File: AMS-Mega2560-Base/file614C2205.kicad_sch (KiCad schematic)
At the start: 5 parts, among them IC1 CD74HC4050ME4, IC2 CD74HC4050ME4, J6 Conn_01x03, J7 Conn_01x08

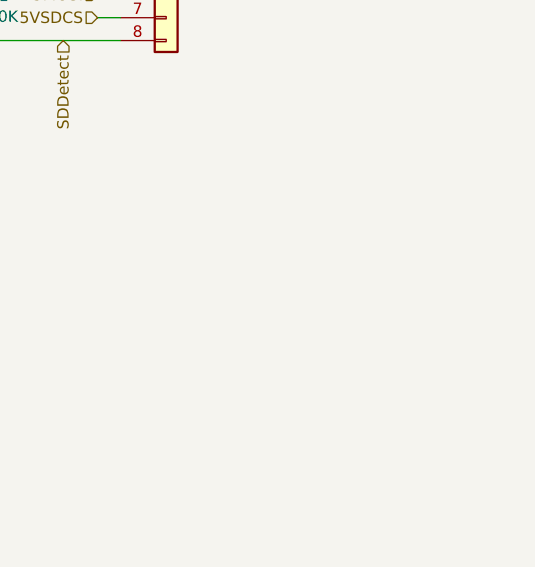
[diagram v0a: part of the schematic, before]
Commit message: BaseBoard fixes and updates. doing schematic work.
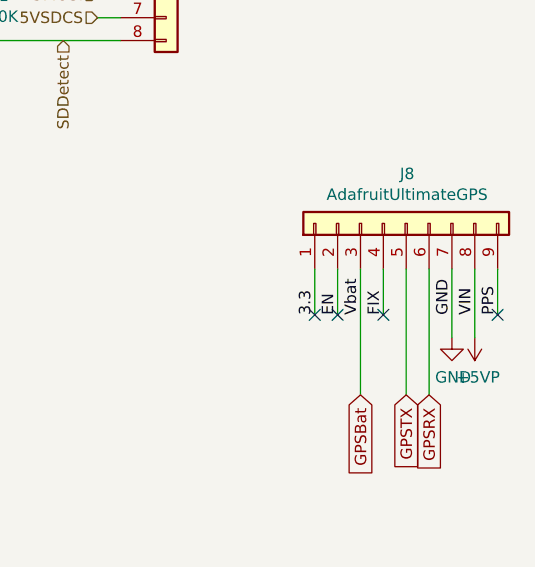
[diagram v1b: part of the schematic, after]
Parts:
- added J8: AdafruitUltimateGPS, Connector_PinSocket_2.54mm:PinSocket_1x09_P2.54mm_Vertical, symbol Connector_Generic:Conn_01x09
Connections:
- net +5VP: now also J8.8 (Pin_8)
- net GND: now also J8.7 (Pin_7)
- new net 3.3: J8.1 (Pin_1)
- new net EN: J8.2 (Pin_2)
- new net FIX: J8.4 (Pin_4)
- new net GPSBat: J8.3 (Pin_3)
- new net GPSRX: J8.6 (Pin_6)
- new net GPSTX: J8.5 (Pin_5)
- new net PPS: J8.9 (Pin_9)
- no-connect marks 7 -> 11
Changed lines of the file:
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@@
   (no_connect (at 205.74 59.69))
   (no_connect (at 81.28 45.72))
+  (no_connect (at 247.65 105.41))
   (no_connect (at 81.28 118.11))
+  (no_connect (at 227.33 105.41))
   (no_connect (at 81.28 110.49))
   (no_connect (at 81.28 38.1))
+  (no_connect (at 234.95 105.41))
+  (no_connect (at 229.87 105.41))
   (wire (pts (xy 49.53 107.95) (xy 53.34 107.95))
     (stroke (width 0) (type default) (color 0 0 0 0))
   )
+  (wire (pts (xy 227.33 105.41) (xy 227.33 100.33))
+    (stroke (width 0) (type default) (color 0 0 0 0))
+  )
   (wire (pts (xy 200.66 62.23) (xy 205.74 62.23))
     (stroke (width 0) (type default) (color 0 0 0 0))
@@
     (stroke (width 0) (type default) (color 0 0 0 0))
   )
+  (wire (pts (xy 237.49 100.33) (xy 237.49 114.3))
+    (stroke (width 0) (type default) (color 0 0 0 0))
+  )
   (wire (pts (xy 86.36 113.03) (xy 81.28 113.03))
     (stroke (width 0) (type default) (color 0 0 0 0))
@@
     (stroke (width 0) (type default) (color 0 0 0 0))
   )
+  (wire (pts (xy 232.41 100.33) (xy 232.41 114.3))
+    (stroke (width 0) (type default) (color 0 0 0 0))
+  )
   (wire (pts (xy 53.34 40.64) (xy 50.8 40.64))
     (stroke (width 0) (type default) (color 0 0 0 0))
@@
     (stroke (width 0) (type default) (color 0 0 0 0))
   )
+  (wire (pts (xy 247.65 105.41) (xy 247.65 100.33))
+    (stroke (width 0) (type default) (color 0 0 0 0))
+  )
   (wire (pts (xy 205.74 57.15) (xy 204.47 57.15))
     (stroke (width 0) (type default) (color 0 0 0 0))
@@
     (stroke (width 0) (type default) (color 0 0 0 0))
   )
+  (wire (pts (xy 240.03 100.33) (xy 240.03 114.3))
+    (stroke (width 0) (type default) (color 0 0 0 0))
+  )
   (wire (pts (xy 53.34 102.87) (xy 53.34 97.79))
     (stroke (width 0) (type default) (color 0 0 0 0))
   )
+  (wire (pts (xy 242.57 107.95) (xy 242.57 100.33))
+    (stroke (width 0) (type default) (color 0 0 0 0))
+  )
+  (wire (pts (xy 245.11 107.95) (xy 245.11 100.33))
+    (stroke (width 0) (type default) (color 0 0 0 0))
+  )
   (wire (pts (xy 50.8 48.26) (xy 53.34 48.26))
     (stroke (width 0) (type default) (color 0 0 0 0))
@@
     (stroke (width 0) (type default) (color 0 0 0 0))
   )
+  (wire (pts (xy 229.87 105.41) (xy 229.87 100.33))
+    (stroke (width 0) (type default) (color 0 0 0 0))
+  )
   (wire (pts (xy 85.09 50.8) (xy 81.28 50.8))
     (stroke (width 0) (type default) (color 0 0 0 0))
   )
+  (wire (pts (xy 234.95 105.41) (xy 234.95 100.33))
+    (stroke (width 0) (type default) (color 0 0 0 0))
+  )
   (wire (pts (xy 96.52 101.6) (xy 102.87 101.6))
     (stroke (width 0) (type default) (color 0 0 0 0))
+  )
+  (label "GND" (at 242.57 105.41 90)
+    (effects (font (size 1.27 1.27)) (justify left bottom))
+  )
+  (label "VIN" (at 245.11 105.41 90)
+    (effects (font (size 1.27 1.27)) (justify left bottom))
+  )
+  (label "FIX" (at 234.95 105.41 90)
+    (effects (font (size 1.27 1.27)) (justify left bottom))
+  )
+  (label "PPS" (at 247.65 105.41 90)
+    (effects (font (size 1.27 1.27)) (justify left bottom))
+  )
+  (label "Vbat" (at 232.41 105.41 90)
+    (effects (font (size 1.27 1.27)) (justify left bottom))
+  )
+  (label "EN" (at 229.87 105.41 90)
+    (effects (font (size 1.27 1.27)) (justify left bottom))
+  )
+  (label "3.3" (at 227.33 105.41 90)
+    (effects (font (size 1.27 1.27)) (justify left bottom))
+  )
+  (global_label "GPSTX" (shape input) (at 237.49 114.3 270) (fields_autoplaced)
+    (effects (font (size 1.27 1.27)) (justify right))
+    (property "Intersheet References" "${INTERSHEET_REFS}" (id 0) (at 182.88 60.96 0)
+      (effects (font (size 1.27 1.27)) hide)
+    )
+  )
+  (global_label "GPSBat" (shape input) (at 232.41 114.3 270) (fields_autoplaced)
+    (effects (font (size 1.27 1.27)) (justify right))
+    (property "Intersheet References" "${INTERSHEET_REFS}" (id 0) (at 182.88 60.96 0)
+      (effects (font (size 1.27 1.27)) hide)
+    )
+  )
+  (global_label "GPSRX" (shape input) (at 240.03 114.3 270) (fields_autoplaced)
+    (effects (font (size 1.27 1.27)) (justify right))
+    (property "Intersheet References" "${INTERSHEET_REFS}" (id 0) (at 182.88 60.96 0)
+      (effects (font (size 1.27 1.27)) hide)
+    )
   )
   (hierarchical_label "3.3MOSI" (shape input) (at 50.8 45.72 180)
@@
   (symbol (lib_id "power:+3.3V") (at 53.34 33.02 0) (unit 1)
     (in_bom yes) (on_board yes)
-    (property "Reference" "#PWR012" (id 0) (at 53.34 36.83 0)
+    (property "Reference" "#PWR09" (id 0) (at 53.34 36.83 0)
       (effects (font (size 1.27 1.27)) hide)
     )
@@
   (symbol (lib_id "power:GND") (at 53.34 60.96 0) (unit 1)
     (in_bom yes) (on_board yes)
-    (property "Reference" "#PWR013" (id 0) (at 53.34 67.31 0)
+    (property "Reference" "#PWR010" (id 0) (at 53.34 67.31 0)
       (effects (font (size 1.27 1.27)) hide)
     )
@@
   (symbol (lib_id "power:+3.3V") (at 53.34 97.79 0) (unit 1)
     (in_bom yes) (on_board yes)
-    (property "Reference" "#PWR014" (id 0) (at 53.34 101.6 0)
+    (property "Reference" "#PWR011" (id 0) (at 53.34 101.6 0)
       (effects (font (size 1.27 1.27)) hide)
     )
@@
   (symbol (lib_id "power:GND") (at 53.34 125.73 0) (unit 1)
     (in_bom yes) (on_board yes)
-    (property "Reference" "#PWR015" (id 0) (at 53.34 132.08 0)
+    (property "Reference" "#PWR012" (id 0) (at 53.34 132.08 0)
       (effects (font (size 1.27 1.27)) hide)
     )
@@
   (symbol (lib_id "power:GND") (at 200.66 62.23 270) (mirror x) (unit 1)
     (in_bom yes) (on_board yes)
-    (property "Reference" "#PWR018" (id 0) (at 194.31 62.23 0)
+    (property "Reference" "#PWR015" (id 0) (at 194.31 62.23 0)
       (effects (font (size 1.27 1.27)) hide)
     )
@@
   (symbol (lib_id "power:+5VP") (at 204.47 55.88 0) (unit 1)
     (in_bom yes) (on_board yes)
-    (property "Reference" "#PWR019" (id 0) (at 204.47 59.69 0)
+    (property "Reference" "#PWR016" (id 0) (at 204.47 59.69 0)
       (effects (font (size 1.27 1.27)) hide)
     )
@@
   (symbol (lib_id "power:+5VP") (at 189.23 63.5 0) (unit 1)
     (in_bom yes) (on_board yes)
-    (property "Reference" "#PWR017" (id 0) (at 189.23 67.31 0)
+    (property "Reference" "#PWR014" (id 0) (at 189.23 67.31 0)
       (effects (font (size 1.27 1.27)) hide)
     )
@@
   (symbol (lib_id "power:GND") (at 102.87 106.68 0) (unit 1)
     (in_bom yes) (on_board yes)
-    (property "Reference" "#PWR016" (id 0) (at 102.87 113.03 0)
+    (property "Reference" "#PWR013" (id 0) (at 102.87 113.03 0)
       (effects (font (size 1.27 1.27)) hide)
     )
@@
       (effects (font (size 1.27 1.27)) hide)
     )
+    (pin "1")
+  )
+  (symbol (lib_id "Connector_Generic:Conn_01x09") (at 237.49 95.25 90) (unit 1)
+    (in_bom yes) (on_board yes)
+    (property "Reference" "J8" (id 0) (at 237.5916 89.7382 90))
+    (property "Value" "AdafruitUltimateGPS" (id 1) (at 237.5916 92.0496 90))
+    (property "Footprint" "Connector_PinSocket_2.54mm:PinSocket_1x09_P2.54mm_Vertical" (id 2) (at 237.49 95.25 0)
+      (effects (font (size 1.27 1.27)) hide)
+    )
+    (property "Datasheet" "~" (id 3) (at 237.49 95.25 0)
+      (effects (font (size 1.27 1.27)) hide)
+    )
+    (pin "1")
+    (pin "2")
+    (pin "3")
+    (pin "4")
+    (pin "5")
+    (pin "6")
+    (pin "7")
+    (pin "8")
+    (pin "9")
+  )
+  (symbol (lib_id "power:+5VP") (at 245.11 107.95 0) (mirror x) (unit 1)
+    (in_bom yes) (on_board yes)
+    (property "Reference" "#PWR018" (id 0) (at 245.11 104.14 0)
+      (effects (font (size 1.27 1.27)) hide)
+    )
+    (property "Value" "+5VP" (id 1) (at 245.491 112.3442 0))
+    (property "Footprint" "" (id 2) (at 245.11 107.95 0)
+      (effects (font (size 1.27 1.27)) hide)
+    )
+    (property "Datasheet" "" (id 3) (at 245.11 107.95 0)
+      (effects (font (size 1.27 1.27)) hide)
+    )
+    (pin "1")
+  )
+  (symbol (lib_id "power:GND") (at 242.57 107.95 0) (unit 1)
+    (in_bom yes) (on_board yes)
+    (property "Reference" "#PWR017" (id 0) (at 242.57 114.3 0)
+      (effects (font (size 1.27 1.27)) hide)
+    )
+    (property "Value" "GND" (id 1) (at 242.697 112.3442 0))
+    (property "Footprint" "" (id 2) (at 242.57 107.95 0)
+      (effects (font (size 1.27 1.27)) hide)
+    )
+    (property "Datasheet" "" (id 3) (at 242.57 107.95 0)
+      (effects (font (size 1.27 1.27)) hide)
+    )
